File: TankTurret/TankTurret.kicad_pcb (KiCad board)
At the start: 2 copper layers, 35 x 60 mm, 86 parts, among them J1 Conn_01x04_Socket, J2 USB_C_Receptacle_USB2.0_16P, J3 Conn_01x02, J4 Conn_01x02, J5 Conn_01x02, J6 Conn_01x03, Q1 MMBT3904, SW1 SW_Push, SW2 SW_Push, U1 ESP32-S3-WROOM-1, U3 ME6211C28M5G, U4 LN1234B132MR-G

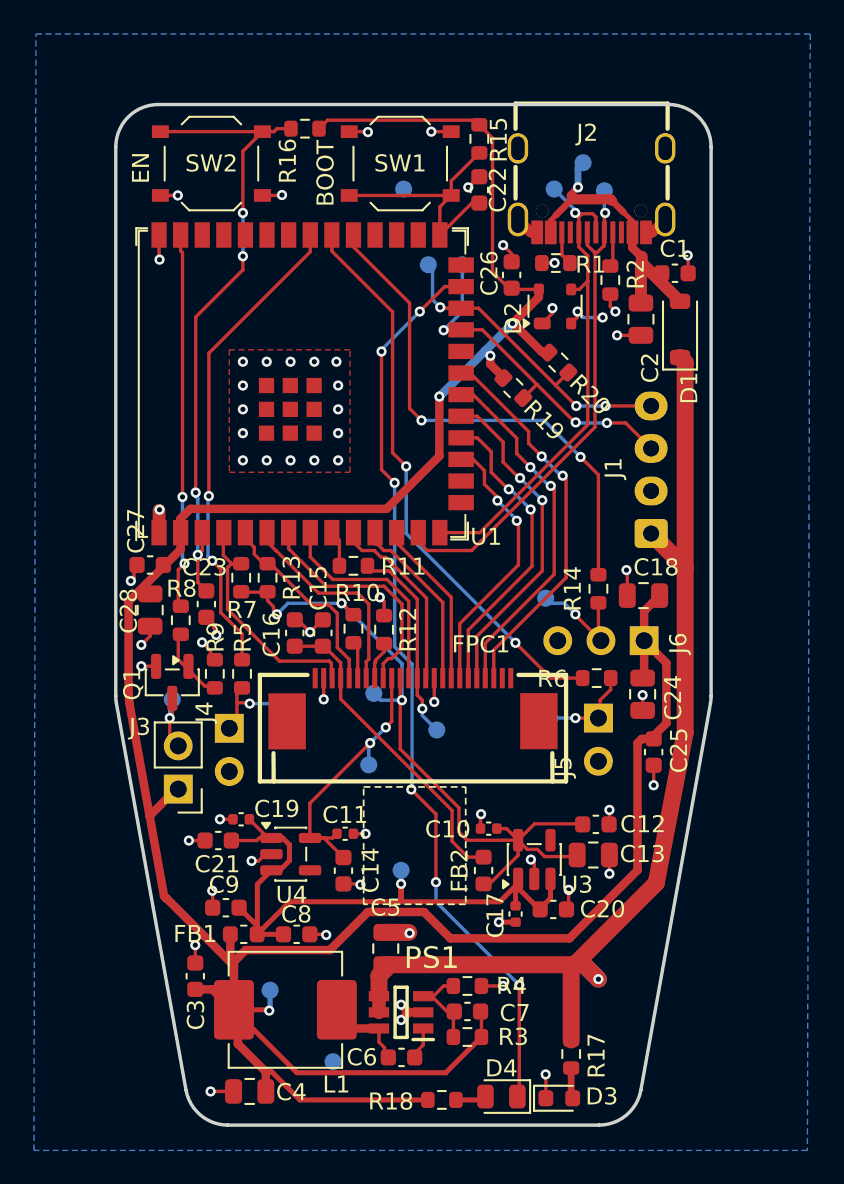
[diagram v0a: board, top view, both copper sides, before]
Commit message: Signed-off-by: SMAUG\Pete <pwbrophy@gmail.com>
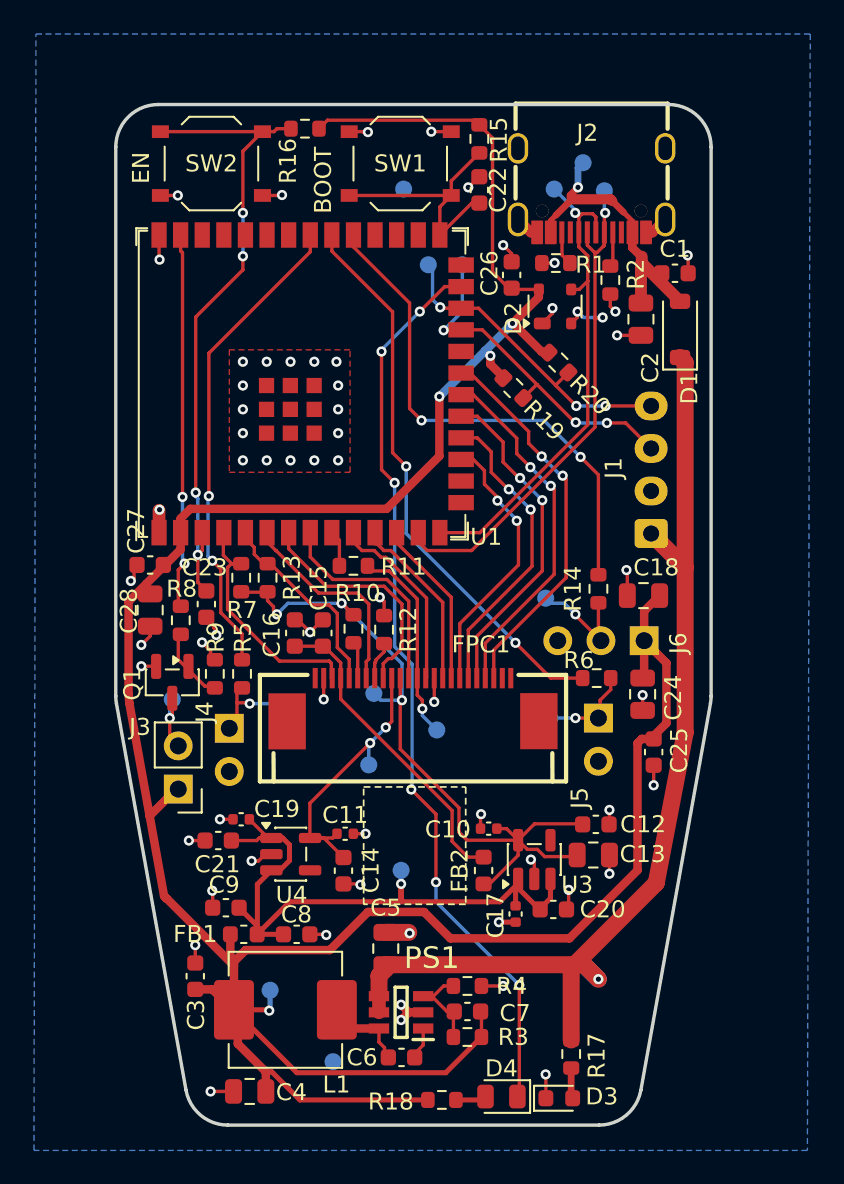
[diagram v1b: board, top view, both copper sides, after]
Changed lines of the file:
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@@
 		(tags "resistor")
 		(property "Reference" "R6"
-			(at 2.6 -0.05 0)
+			(at 1.05 1.05 0)
 			(layer "F.SilkS")
 			(effects
@@
 		(tags "Through hole pin header THT 1x02 2.54mm single row")
 		(property "Reference" "J5"
-			(at 2.05 -2.85 90)
+			(at 1.1 -4.7 90)
 			(layer "F.SilkS")
 			(effects
@@
 	)
 	(gr_text "BOOT"
-		(at 66.75 47.3 90)
+		(at 66.6 47.7 90)
 		(layer "F.SilkS" knockout)
 		(effects
